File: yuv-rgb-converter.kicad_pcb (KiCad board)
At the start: 2 copper layers, 65.3 x 53.1 mm, 56 parts, among them J1 YUV IN, J2 RGB OUT, J3 POWER, Q1 BC548, Q2 BC548, Q3 BC548, Q4 BC548, Q5 BC548, Q6 BC548, Q7 BC548, Q8 BC548, Q9 BC558, U1 4027, U2 4066

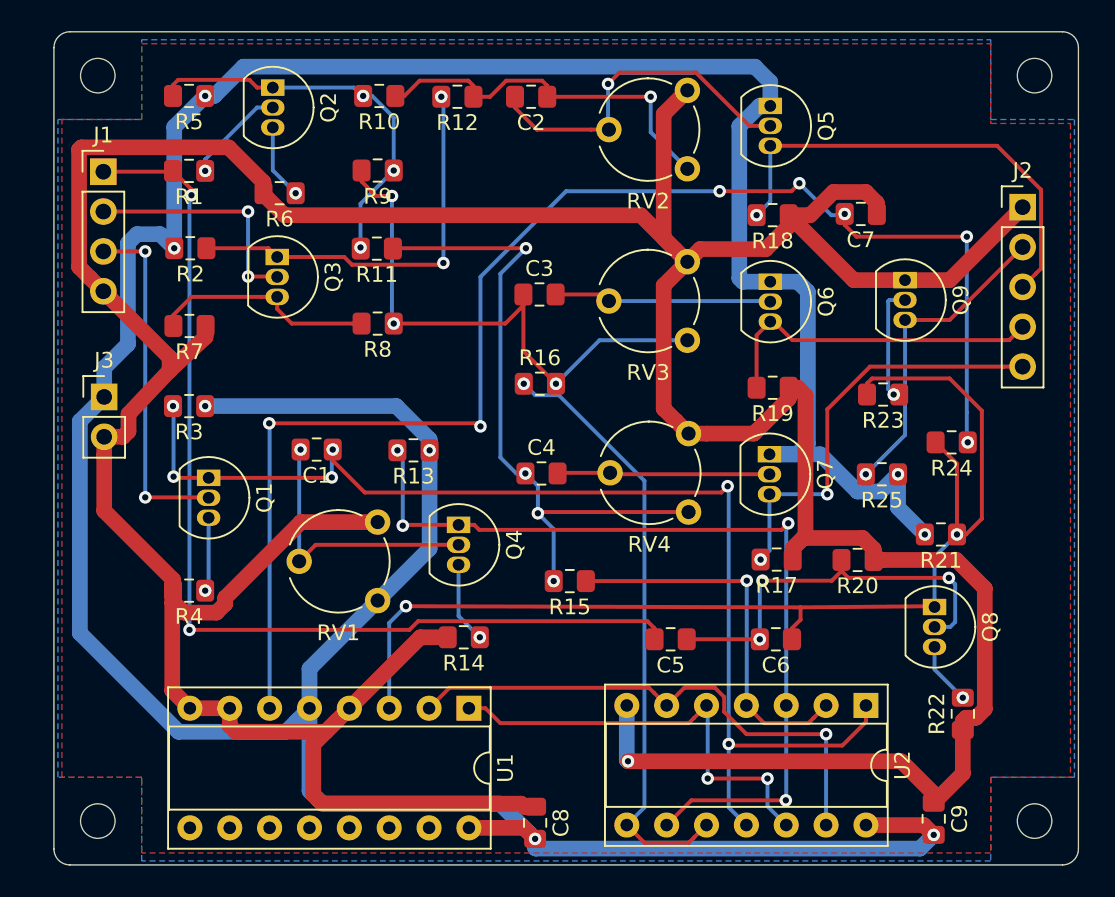
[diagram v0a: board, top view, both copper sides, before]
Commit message: README, original schematics
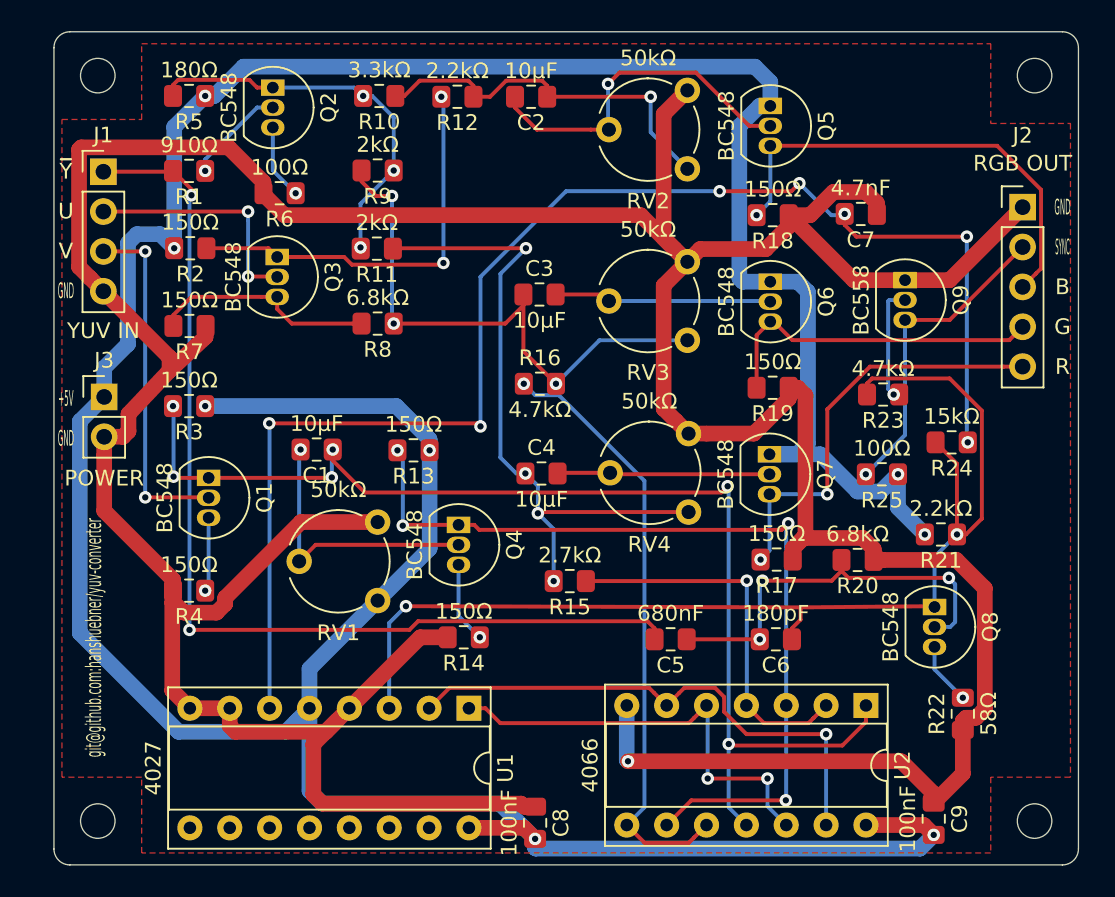
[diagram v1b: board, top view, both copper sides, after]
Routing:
- removed copper zone on B.Cu, net +5V
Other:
- board text added: "+5V"
- board text added: "B"
- board text added: "G"
- board text added: "GND"
- board text added: "R"
- board text added: "SYNC"
- board text added: "U"
- board text added: "V"
- board text added: "git@github.com:hanshuebner/yuv-converter"
- board text added: "~Y"
